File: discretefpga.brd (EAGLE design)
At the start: 61.3 x 61.6 mm, 50 parts, among them IC1 74HC595D, IC10 74HC251D, IC11 74HC595D, IC12 74HC595D, IC13 74HC173D, IC3 74HC251D, IC4 74HC125D, IC5 74HC126D, IC6 4066D, IC7 74HC126D, IC8 74HC125D, IC9 74HC595D

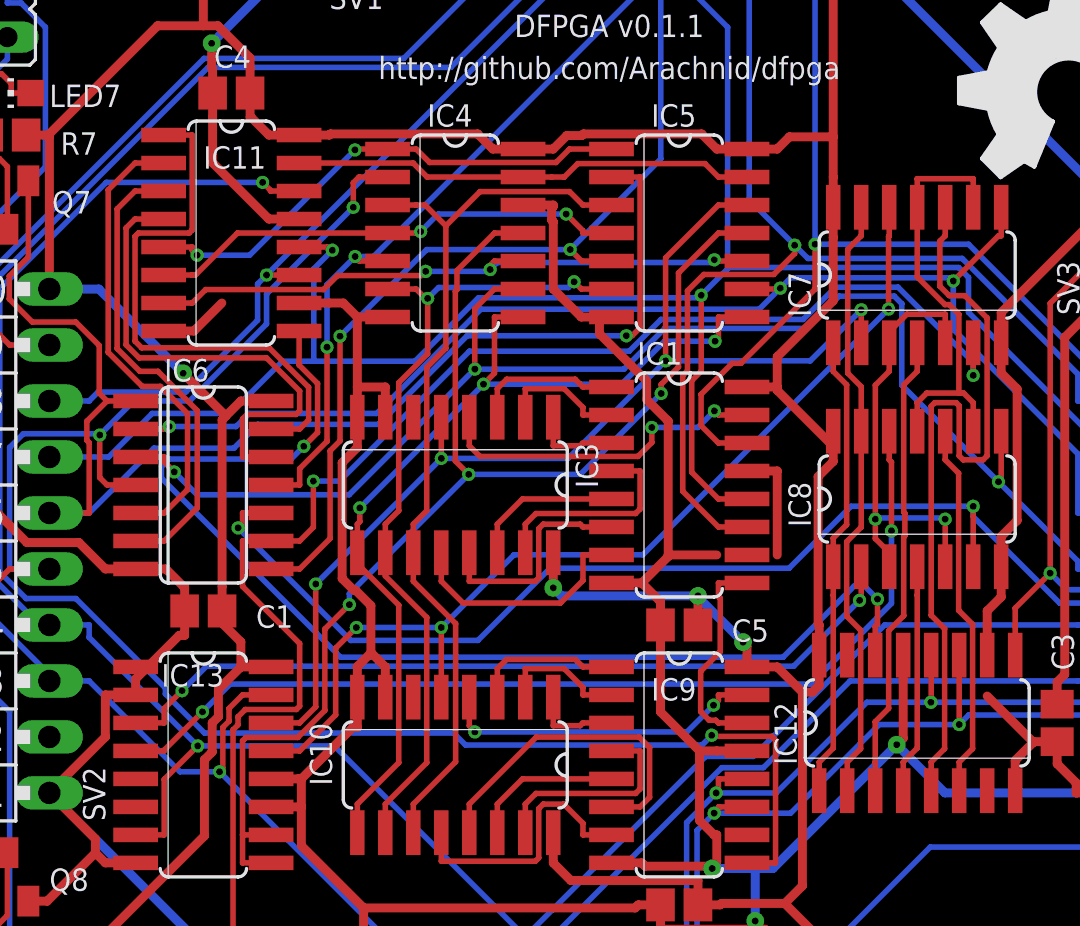
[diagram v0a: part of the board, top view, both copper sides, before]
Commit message: updated schematic
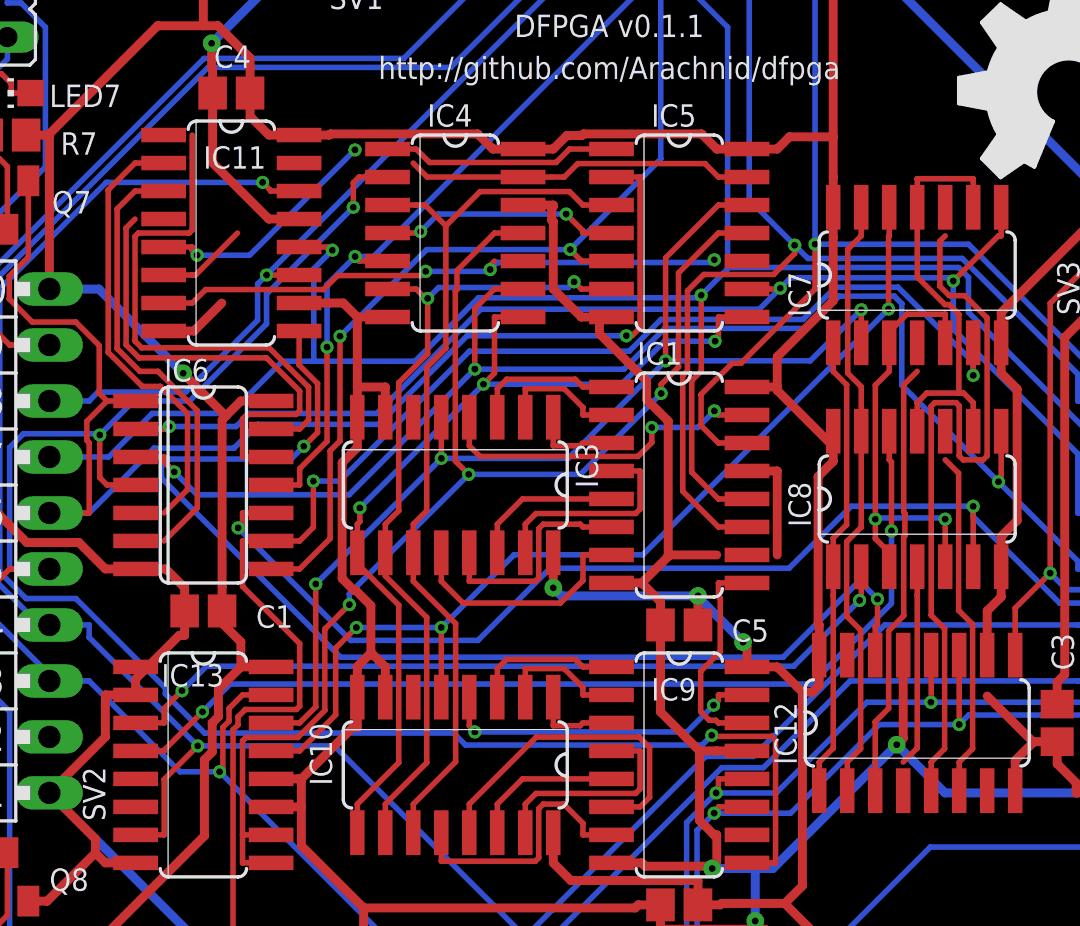
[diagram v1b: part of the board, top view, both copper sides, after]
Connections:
- net A_SEL renamed L0_TO_A/L1_TO_A_E0
- net B_SEL renamed U1_TO_B/U0_TO_B_E0
- net C_SEL renamed R0_TO_C/R1_TO_C_E0
- net EW0_SW renamed L0_TO_R0
- net EW1_SW renamed L1_TO_R1
- net LATCHING renamed LATCHING_E0
- net NS0_SW renamed U1_TO_D1
- net NS1_SW renamed U0_TO_D0
- net O0_S0_EN renamed O0_TO_D1
- net O0_S1_EN renamed O0_TO_D0_E0
- net O1_E0_EN renamed O1_TO_R0
- net O1_E1_EN renamed O1_TO_R1_E0
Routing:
- net U1_TO_B/U0_TO_B_E0: track 21.9 -> 15.1 mm
- net LATCHING_E0: track 21.1 -> 15.9 mm
- net R0_TO_C/R1_TO_C_E0: track 29.1 -> 26.5 mm
- net O1_TO_R0: track 35.7 -> 34.4 mm
- net O0_TO_D1: track 21.2 -> 19.9 mm
- net L0_TO_A/L1_TO_A_E0: track 23.1 -> 21.8 mm
- net U1_TO_D1: track 21.4 -> 20.1 mm
- net U0_TO_D0: track 22.6 -> 21.3 mm
- net O0_TO_D0_E0: track 10.4 -> 9.13 mm
- net L1_TO_R1: track 21.4 -> 20.1 mm
- net L0_TO_R0: track 25.2 -> 23.9 mm
- net O1_TO_R1_E0: track 17.1 -> 15.8 mm
